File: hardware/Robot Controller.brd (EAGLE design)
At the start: 52.4 x 48.9 mm, 18 parts

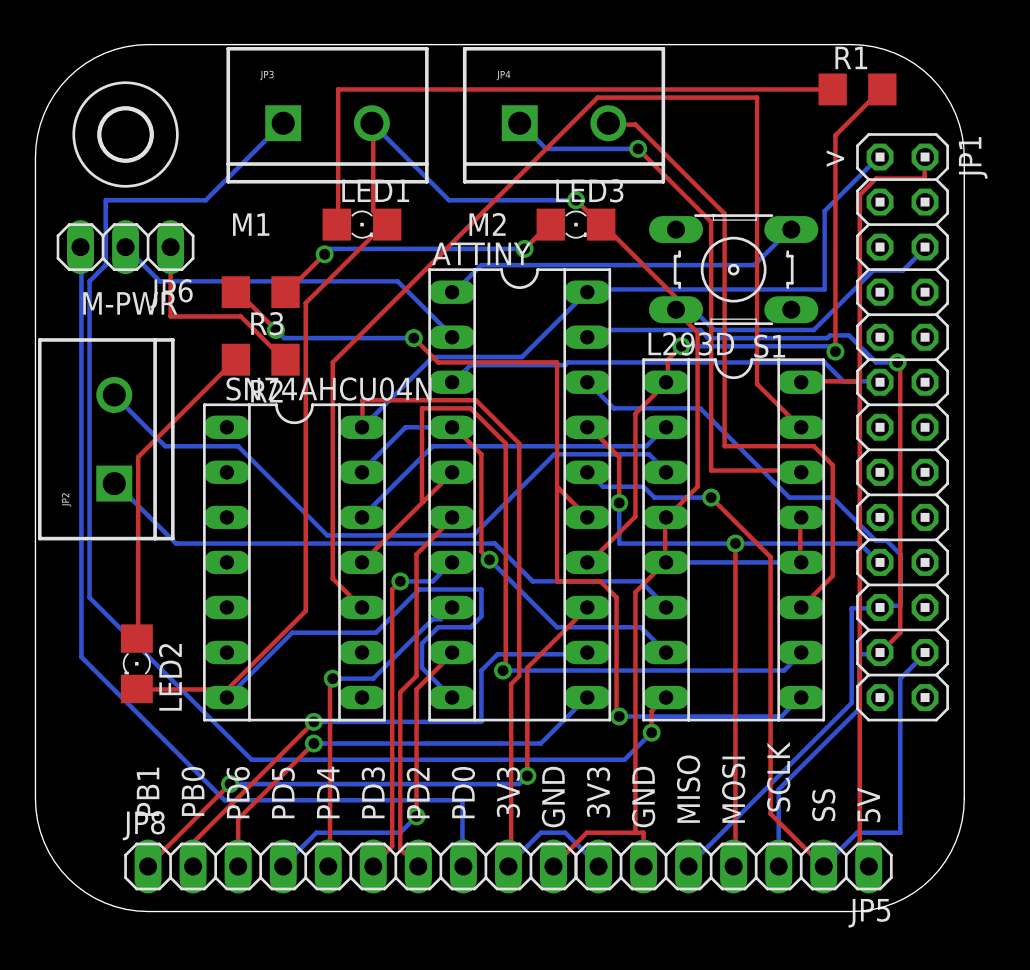
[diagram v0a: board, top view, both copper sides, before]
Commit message: routing
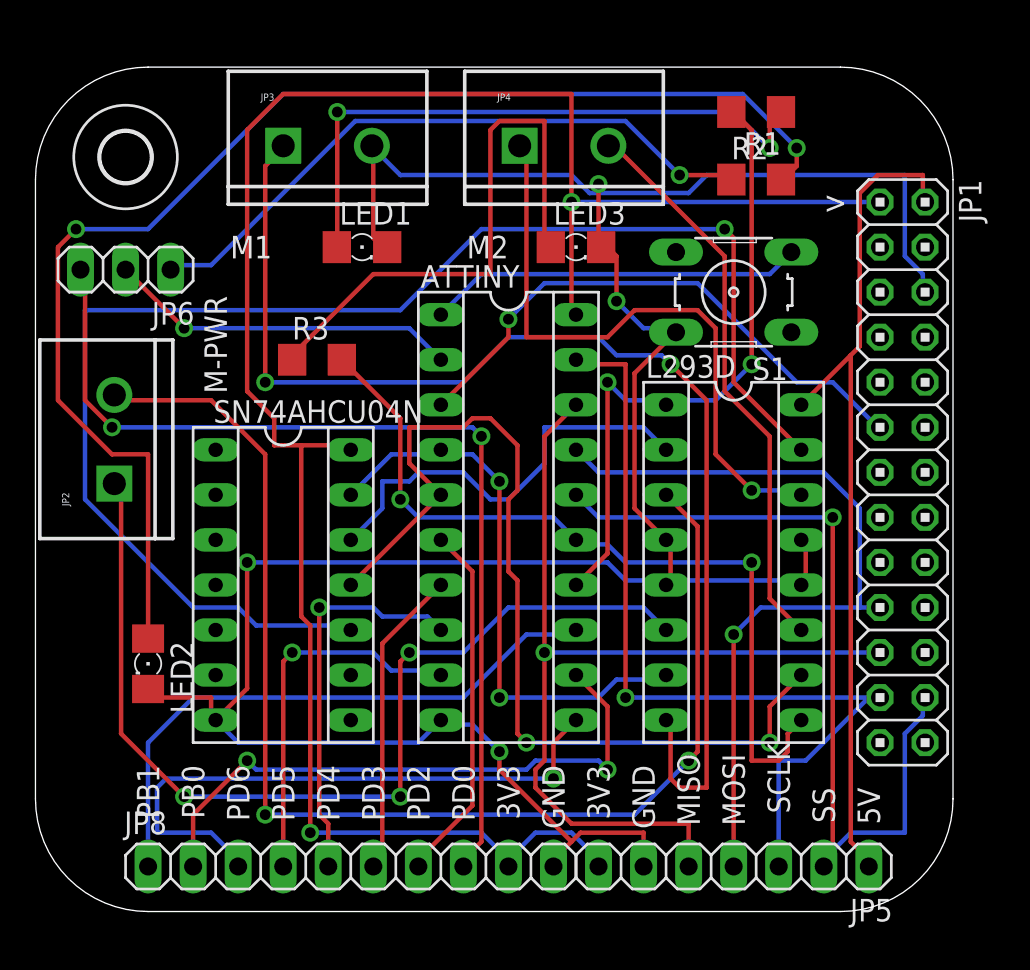
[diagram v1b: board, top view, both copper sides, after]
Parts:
- moved R2 29.7 mm to (82.5, 59.7), turned to 0 degrees
- moved R1 5.85 mm to (82.5, 63.5), turned to 180 degrees
- moved R3 4.96 mm to (57.8, 49.5), turned to 0 degrees
- moved JP1 2.54 mm to (90.8, 43.2)
- moved SN74AHCU04N 1.42 mm to (55.9, 36.8)
- moved ATTINY 1.42 mm to (68.6, 40.6)
- moved JP3 1.27 mm to (55.9, 61.6)
- moved JP4 1.27 mm to (69.2, 61.6)
- moved JP6 1.27 mm to (47.0, 54.6)
- moved H1 1.27 mm to (47.0, 61.0)
- moved L293D 1.27 mm to (81.3, 38.1)
- moved LED1 1.27 mm to (60.3, 55.9)
- moved LED3 1.27 mm to (72.4, 55.9)
- moved S1 1.27 mm to (81.3, 53.3)
- moved LED2 0.63 mm to (48.3, 32.4)
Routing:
- net N$17: track 18.1 -> 74.1 mm, vias 0 -> 2
- net N$8: track 36.7 -> 71.3 mm, vias 0 -> 2
- net VCC: track 80.3 -> 113.3 mm, vias 0 -> 2
- net N$21: track 11.4 -> 36.4 mm, vias 0 -> 1
- net N$9: track 34.0 -> 55.9 mm, vias 0 -> 3
- net N$22: track 64.3 -> 80.9 mm, vias 0 -> 1
- net N$14: track 16.5 -> 32.2 mm, vias 2 -> 0
- net N$11: track 55.7 -> 46.0 mm, vias 3 -> 2
- net N$30: track 25.2 -> 34.5 mm
- net N$6: track 45.7 -> 53.4 mm, vias 0 -> 1
- net N$2: track 25.0 -> 31.6 mm, vias 0 -> 1
- net N$20: track 48.2 -> 54.3 mm, vias 1 -> 2
- net N$13: track 26.7 -> 32.3 mm, vias 1 -> 2
- net N$19: track 37.1 -> 32.0 mm
- net N$15: track 19.3 -> 24.3 mm
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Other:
- board size 52.4 x 48.9 mm -> 51.7 x 47.6 mm
- board text added: "1. A robot may not injure a human being or, through inaction, allow a human being to come to harm. 2. A robot must obey the orders given to it by human beings, except where such orders would conflict with the First Law. 3. A robot must protect its own existence as long as such p rotection does not conflict with the First or Second Laws."

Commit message: tighten up PCB
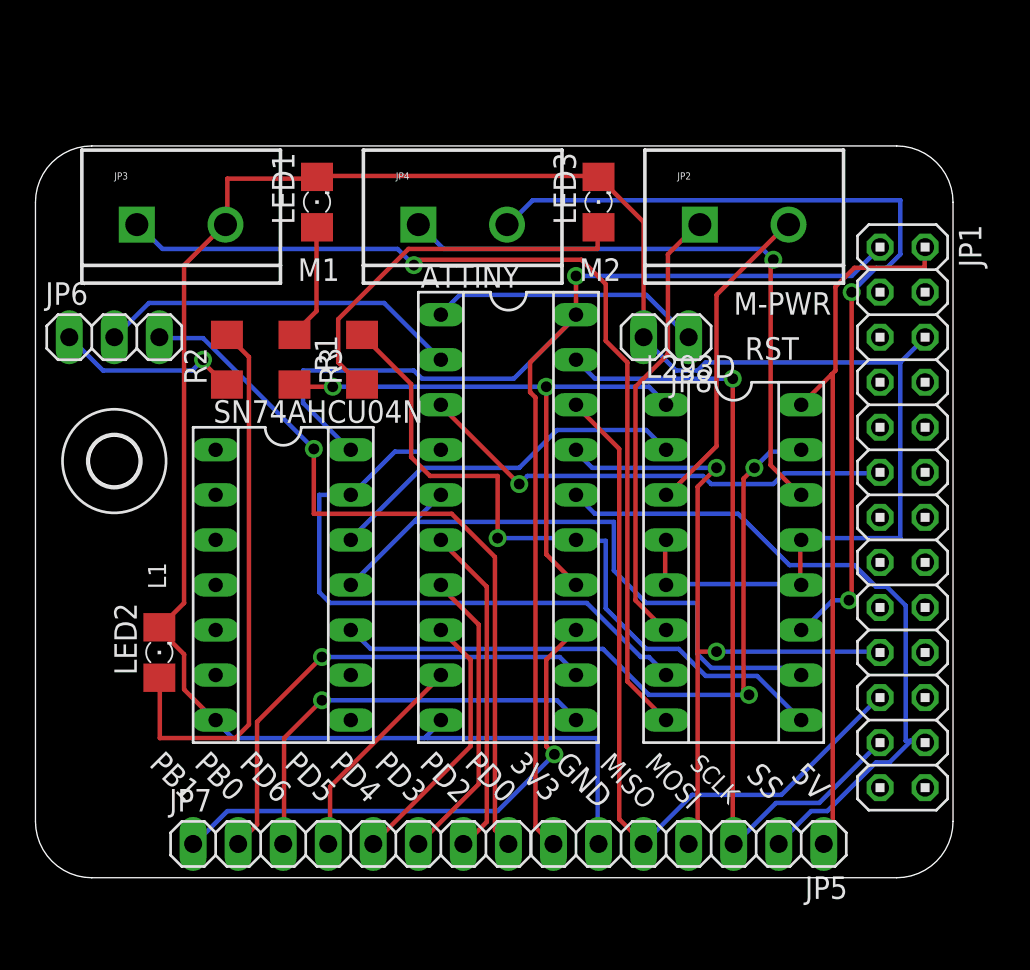
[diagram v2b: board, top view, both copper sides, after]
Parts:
- removed S1: (no value), switch-omron:B3F-10XX
- added JP7: (no value), pinhead:1X08
- JP8: device pinhead:1X10 -> pinhead:1X02
- moved JP2 36.1 mm to (79.4, 57.1), turned to 0 degrees
- moved JP8 34.7 mm to (77.5, 50.8), turned to 180 degrees
- moved R2 31.5 mm to (52.7, 49.5), turned to 90 degrees
- moved R1 29.5 mm to (56.5, 49.5), turned to 270 degrees
- moved H1 17.2 mm to (46.4, 43.8)
- moved JP3 9.38 mm to (47.6, 57.1)
- moved JP4 7.24 mm to (63.5, 57.1)
- moved JP6 3.86 mm to (46.4, 50.8), turned to 0 degrees
- moved LED1 3.59 mm to (57.8, 58.4), turned to 90 degrees
- moved JP5 2.84 mm to (78.7, 22.2)
- moved LED3 2.84 mm to (73.7, 58.4), turned to 90 degrees
- moved R3 2.54 mm to (60.3, 49.5), turned to 90 degrees
- moved JP1 2.54 mm to (90.8, 40.6)
- moved LED2 0.90 mm to (48.9, 33.0), turned to 90 degrees
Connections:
- net GND: now also JP8.2; no longer JP8.10, S1.2
- net N$23: now also JP7.8; no longer JP8.8
- net N$24: now also JP7.7; no longer JP8.7
- net N$25: now also JP7.6; no longer JP8.6
- net N$26: now also JP7.5; no longer JP8.5
- net N$27: now also JP7.4; no longer JP8.4
- net N$28: now also JP7.1; no longer JP8.1
- net N$29: now also JP7.2; no longer JP8.2
- net N$30: now also JP7.3; no longer JP8.3
- net N$31: now also JP8.1; no longer S1.3
- net VCC: no longer JP8.9
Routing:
- net N$8: track 71.3 -> 18.2 mm, vias 2 -> 0
- net N$17: track 74.1 -> 31.2 mm, vias 2 -> 0
- net N$22: track 80.9 -> 40.2 mm, vias 1 -> 2
- net VCC: track 113.3 -> 74.3 mm, vias 2 -> 1
- net N$9: track 55.9 -> 25.2 mm, vias 3 -> 0
- net N$3: track 35.2 -> 6.60 mm, vias 2 -> 0
- net N$21: track 36.4 -> 10.6 mm
- net N$20: track 54.3 -> 35.9 mm, vias 2 -> 0
- net N$19: track 32.0 -> 50.2 mm, vias 0 -> 2
- net GND: track 155.4 -> 139.8 mm, vias 4 -> 0
- net N$10: track 68.7 -> 54.3 mm, vias 2 -> 1
- net N$23: track 55.3 -> 42.7 mm, vias 2 -> 1
- net N$30: track 34.5 -> 23.8 mm
- net N$14: track 32.2 -> 21.8 mm
- net N$6: track 53.4 -> 43.1 mm, vias 1 -> 0
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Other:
- board size 51.7 x 47.6 mm -> 51.7 x 41.3 mm
- board text added: "L1"
- board text added: "RST"
- board text added: "robot core rev 0.1"
- board text removed: "1. A robot may not injure a human being or, through inaction, allow a human being to come to harm. 2. A robot must obey the orders given to it by human beings, except where such orders would conflict with the First Law. 3. A robot must protect its own existence as long as such p rotection does not conflict with the First or Second Laws."
- board text removed: "robot core"
